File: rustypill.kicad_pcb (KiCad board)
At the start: 2 copper layers, 69 x 48 mm, 49 parts, among them IC1 DS3231, J1 USB, J2 PROG, J3 GPIOB, J4 GPIOA, J5 LCD1602, J6 IDC_10P, M2 MountingHole_2.7mm_M2.5, M3 MountingHole_2.7mm_M2.5, M4 MountingHole_2.7mm_M2.5, SW1 Reset, U1 AMS1117-3.3, U2 AT24C512C-SSHD-T, U3 ESP-12F, U4 STM32F103C8Tx, Y1 8MHz

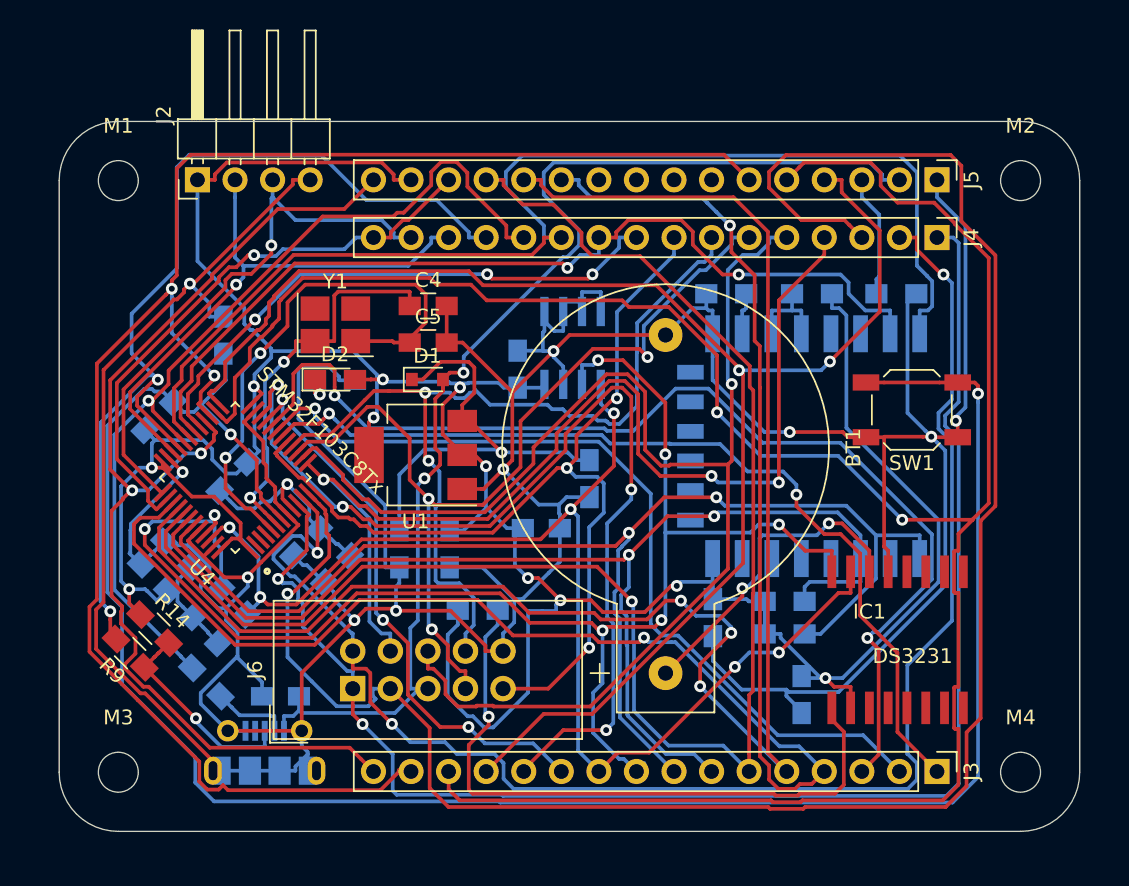
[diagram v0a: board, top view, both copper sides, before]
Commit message: finish pcb design
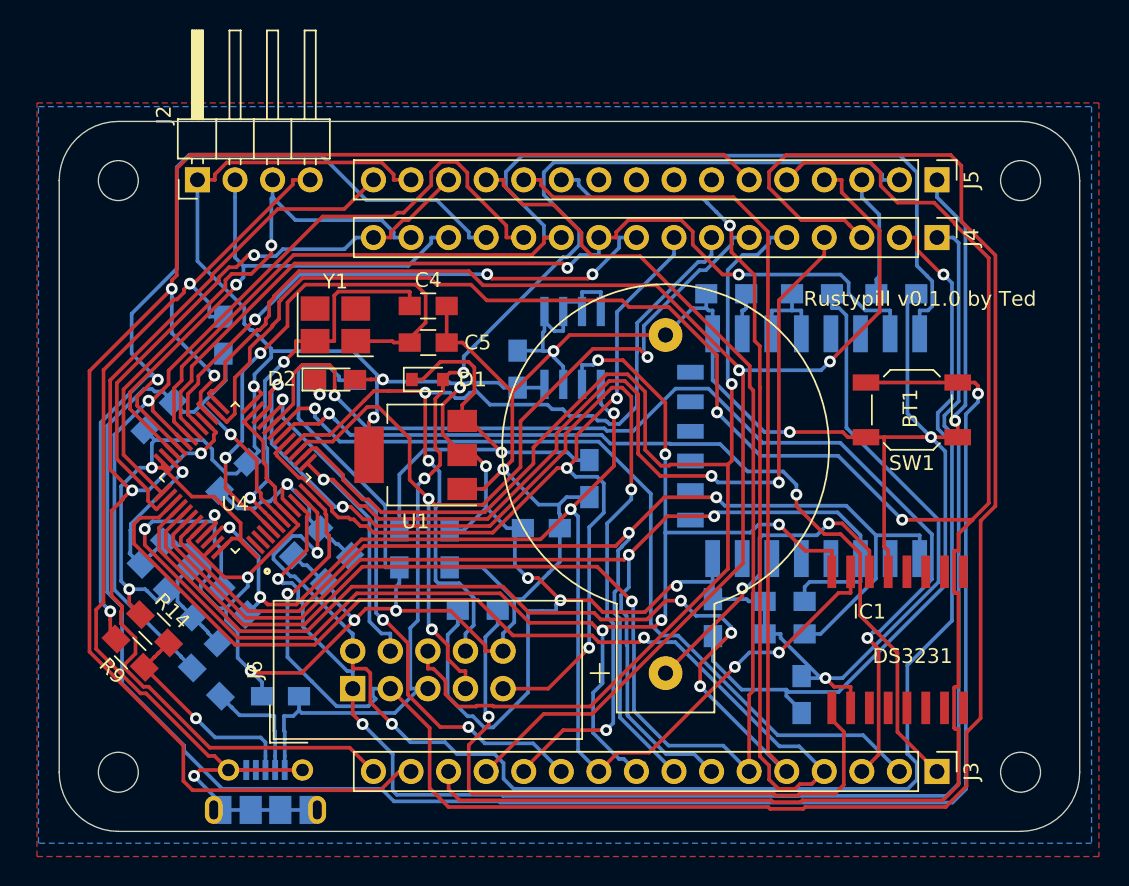
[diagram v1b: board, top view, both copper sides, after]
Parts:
- moved J1 2.65 mm to (82.0, 138.2)
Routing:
- net GND: track 349.5 -> 344.7 mm, vias 10 -> 12
- net USB_DM: track 5.20 -> 7.87 mm
- net VPP: track 79.9 -> 82.6 mm
- net USB_DP: track 13.9 -> 14.7 mm
- net Net-(C6-Pad1): track 137.3 -> 136.5 mm
- added copper zone on B.Cu, net GND
- added copper zone on F.Cu, net GND
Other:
- board text added: "Rustypill v0.1.0 by Ted"

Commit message: finish v0.1.0
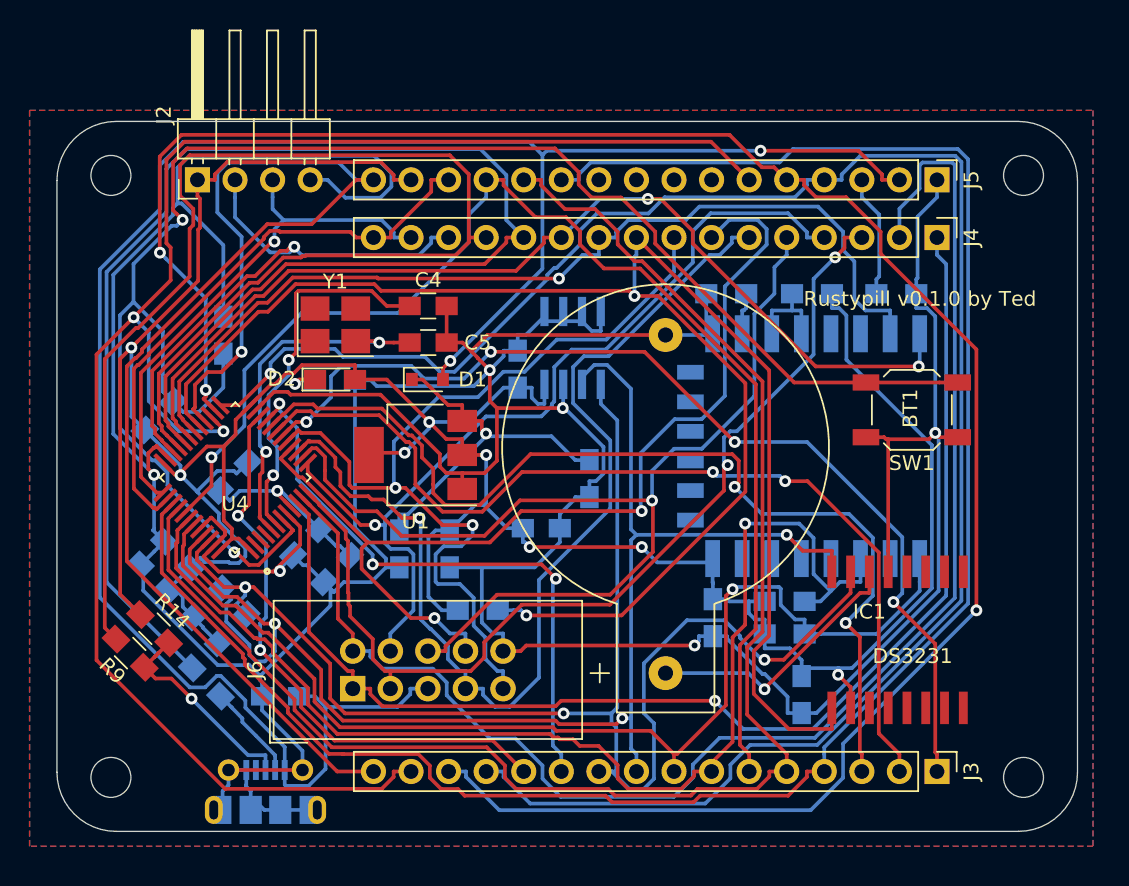
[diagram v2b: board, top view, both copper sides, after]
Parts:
- moved  M1 0.61 mm to (71.5, 95.7)
- moved M3 0.61 mm to (71.5, 136.3)
- moved M2 0.40 mm to (133.2, 95.7)
- moved M4 0.40 mm to (133.2, 136.3)
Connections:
- J4 pad 9: A8 -> 32KHZ_IN
- U4 pad 29: A8 -> 32KHZ_IN
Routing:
- net 32KHZ_IN: track 44.5 -> 121.0 mm, vias 1 -> 2
- net A2: track 134.1 -> 66.1 mm, vias 1 -> 2
- net VPP: track 82.6 -> 138.4 mm
- net A11: track 61.1 -> 100.0 mm, vias 1 -> 0
- net A8: track 38.1 -> 0.00 mm, vias 3 -> 0
- net B11: track 68.3 -> 39.3 mm, vias 4 -> 2
- net B12: track 103.4 -> 129.3 mm, vias 2 -> 1
- net A12: track 66.6 -> 91.5 mm, vias 2 -> 0
- net Net-(C6-Pad1): track 136.5 -> 113.8 mm
- net B5: track 107.4 -> 86.5 mm
- net A4: track 92.9 -> 72.6 mm
- net A0: track 102.2 -> 84.3 mm, vias 2 -> 1
- net B3: track 116.3 -> 132.7 mm, vias 2 -> 0
- net B13: track 158.7 -> 143.3 mm, vias 2 -> 3
- net B15: track 73.6 -> 88.7 mm, vias 2 -> 1
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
